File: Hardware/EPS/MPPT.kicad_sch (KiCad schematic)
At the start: 34 parts

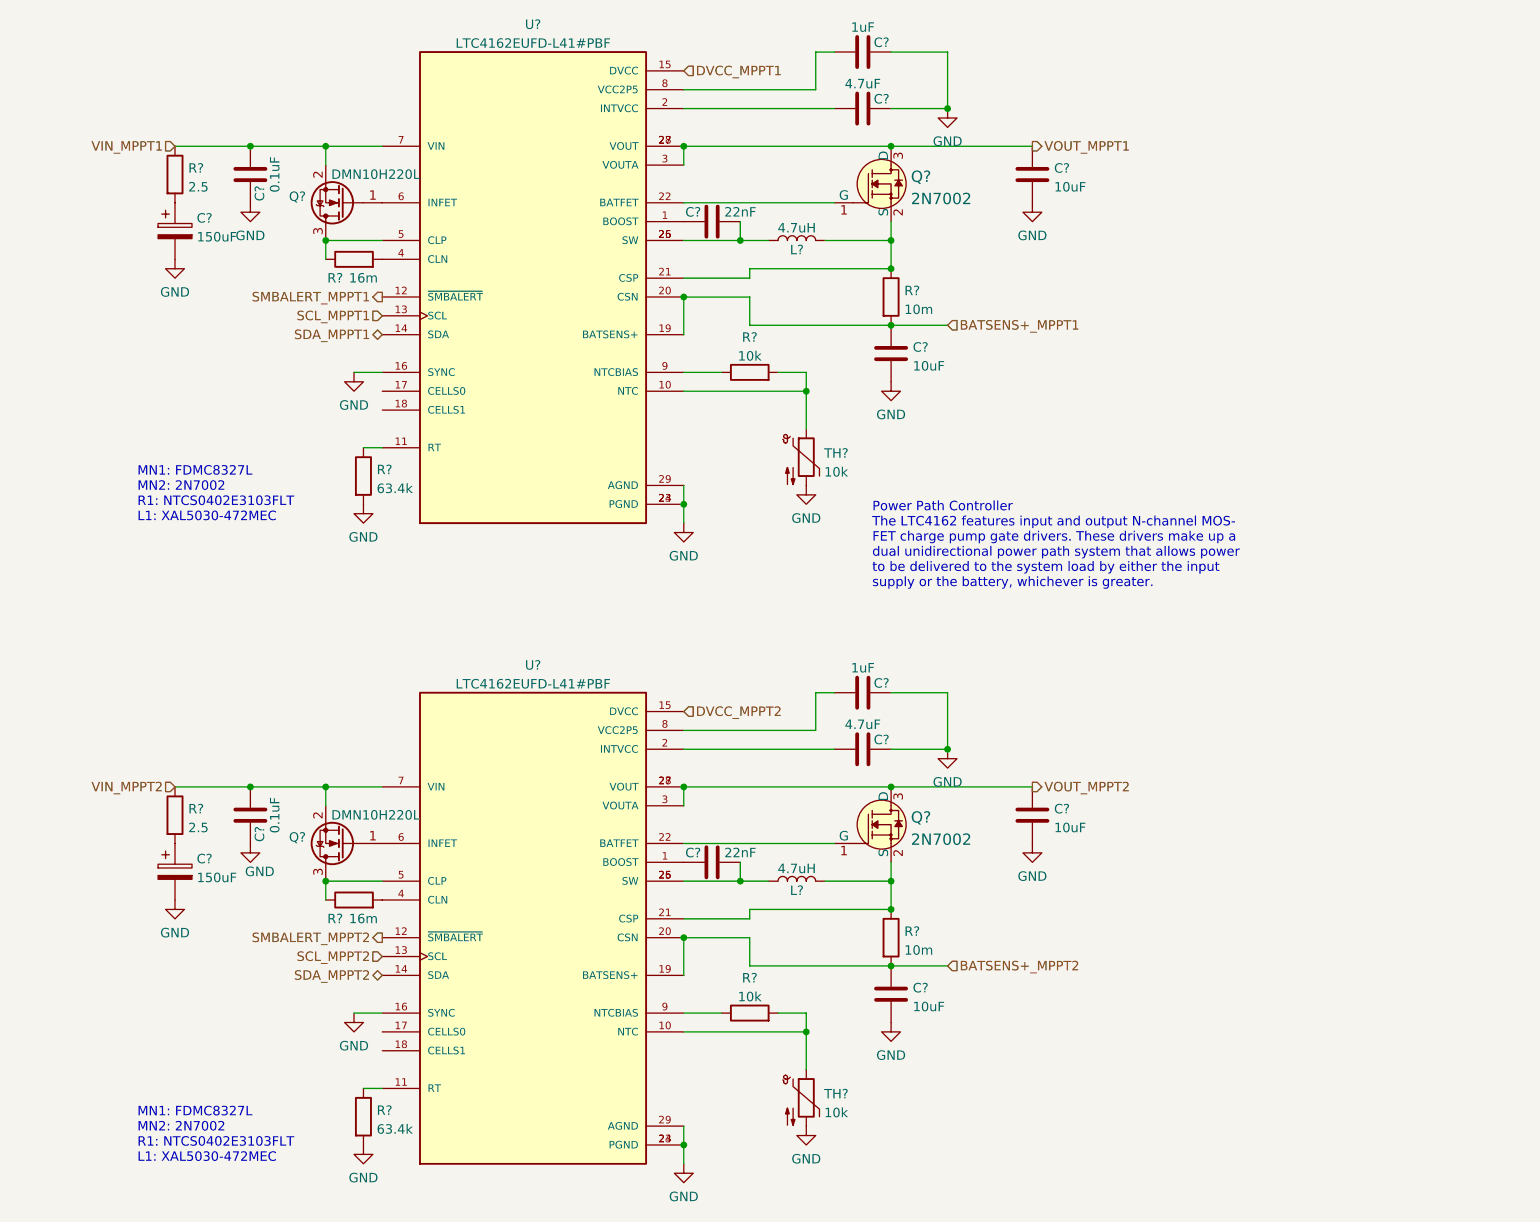
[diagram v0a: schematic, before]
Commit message: EPS v0.0.1
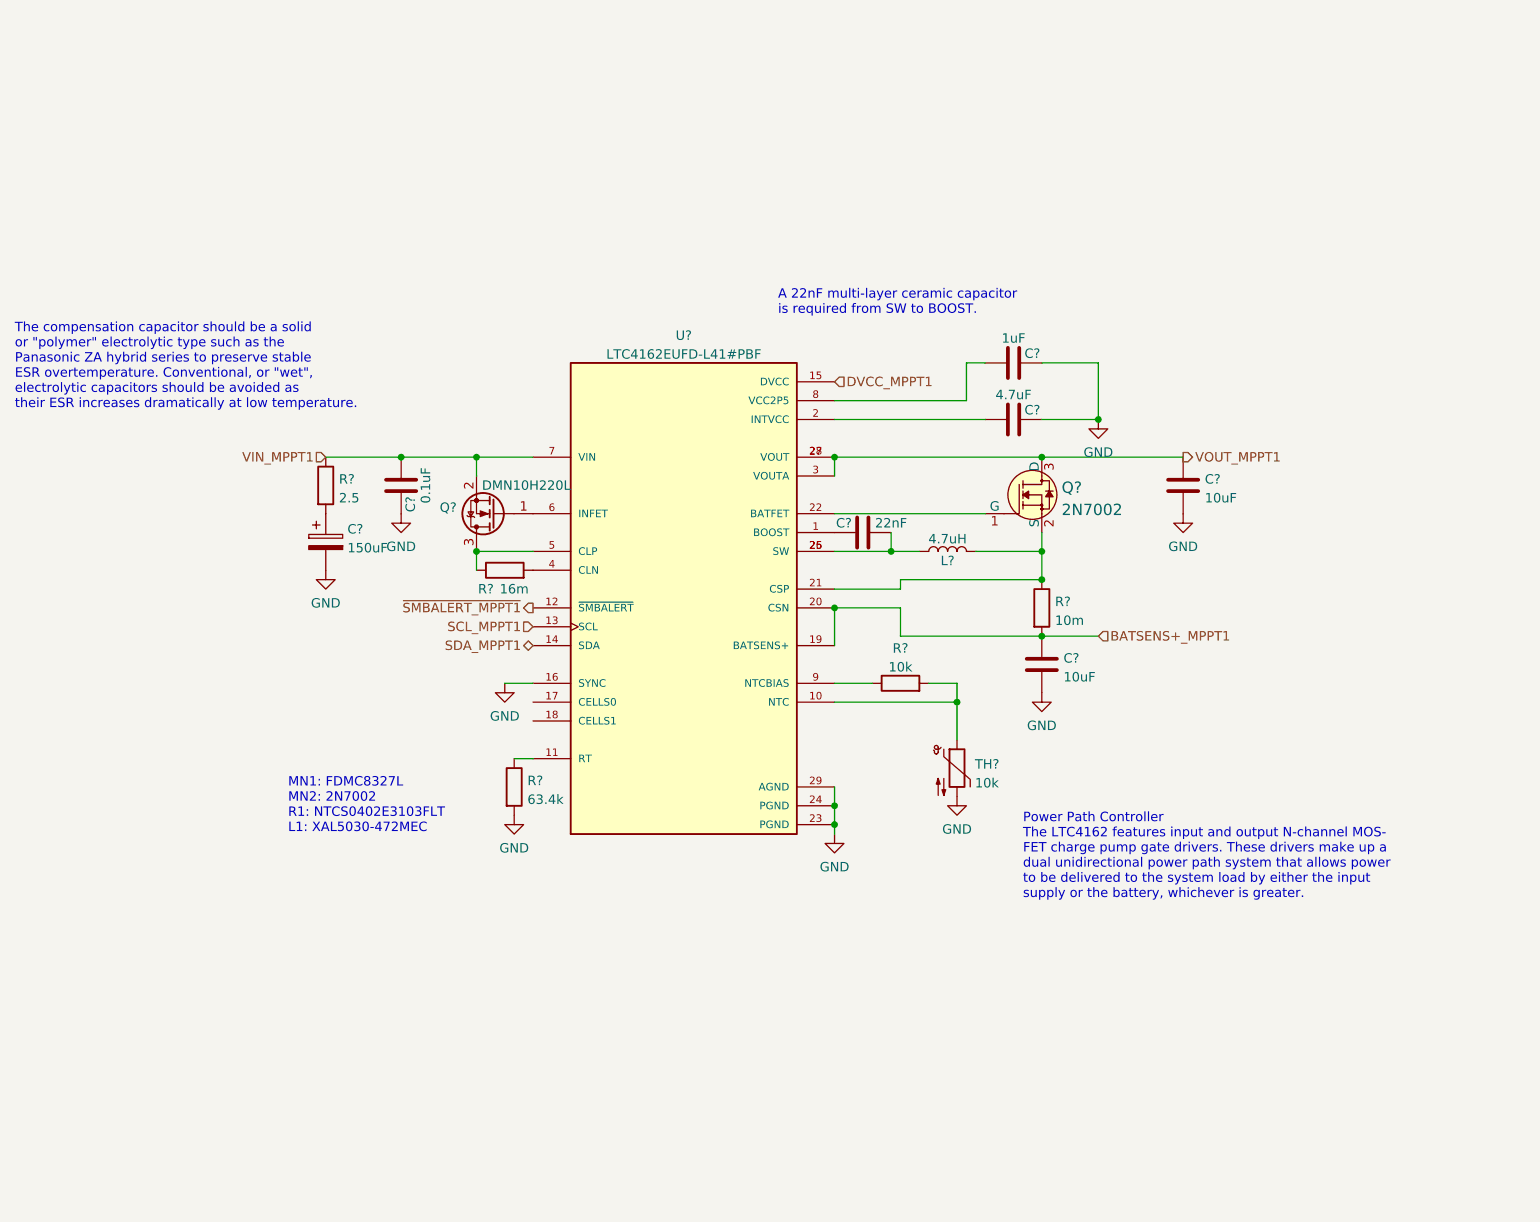
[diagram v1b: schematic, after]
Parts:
- removed C?: 22nF, symbol Device:C
- removed C?: 150uF, symbol Device:C_Polarized
- removed C? (x2): 10uF, symbol Device:C
- removed C?: 4.7uF, symbol Device:C
- removed C?: 1uF, symbol Device:C
- removed C?: 0.1uF, symbol Device:C
- removed L?: 4.7uH, symbol Device:L
- removed Q?: 2N7002, digikey-footprints:SOT-23-3, symbol dk_Transistors-FETs-MOSFETs-Single:2N7002
- removed Q?: DMN10H220L, Package_TO_SOT_SMD:SOT-23, symbol Transistor_FET:DMN10H220L
- removed R?: 10m, symbol Device:R
- removed R?: 16m, symbol Device:R
- removed R?: 63.4k, symbol Device:R
- removed R?: 10k, symbol Device:R
- removed R?: 2.5, symbol Device:R
- removed TH?: 10k, symbol Device:Thermistor_NTC
- removed U?: LTC4162EUFD-L41#PBF, QFN50P500X400X80-29N, symbol LTC4162EUFD-L41_PBF:LTC4162EUFD-L41#PBF
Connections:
- net SMBALERT_MPPT1 renamed ~{SMBALERT_MPPT1}
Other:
- note added: "A 22nF multi-layer ceramic capacitor is required from SW to BOOST."
- note added: "The compensation capacitor should be a solid or "polymer" electrolytic type such as the Panasonic ZA hybrid series to preserve stable ESR overtemperature. Conventional, or "wet", electrolytic capacitors should be avoided as their ESR increases dramatically at low temperature."
- moved on the sheet: C?, L?, Q?, R?, TH?
